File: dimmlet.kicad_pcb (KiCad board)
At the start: 2 copper layers, 204 x 20 mm, 23 parts, among them J1 Conn_01x02, J2 Conn_01x02, J3 CONN288_2-2308107-0_TEC, J4 Conn_01x06, J5 Conn_01x02, J6 Conn_01x02, J7 CONN288_2-2308107-0_TEC, U1 ‎TXS0102, U2 ‎MIC5365-2.5YC5-TR

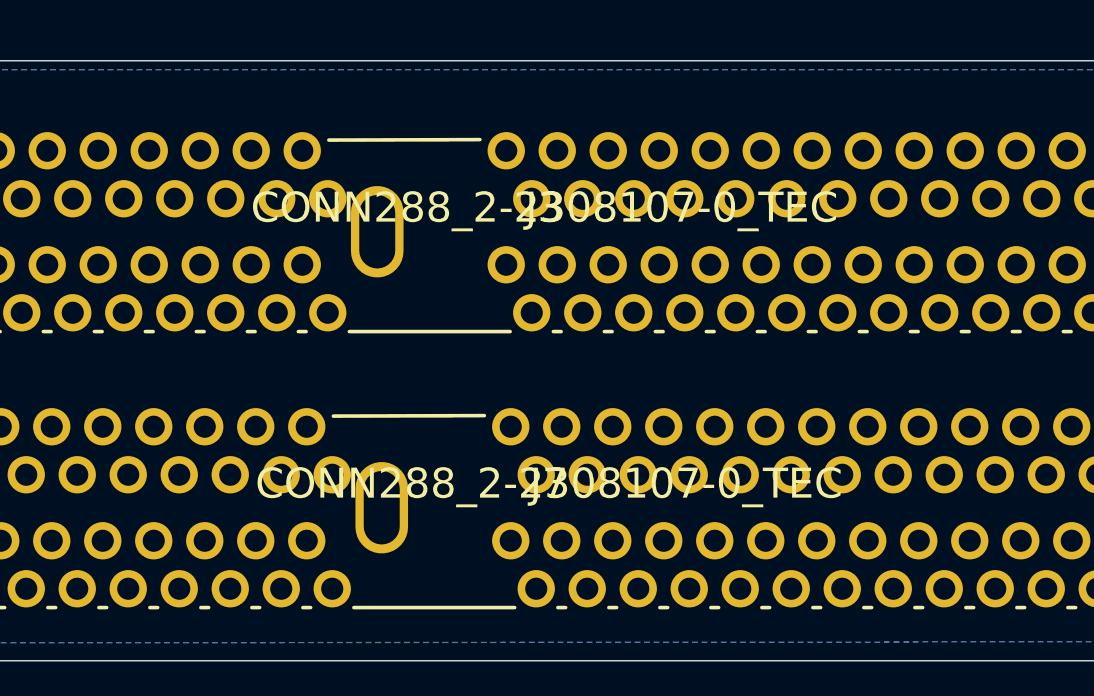
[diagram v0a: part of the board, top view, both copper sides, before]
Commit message: update
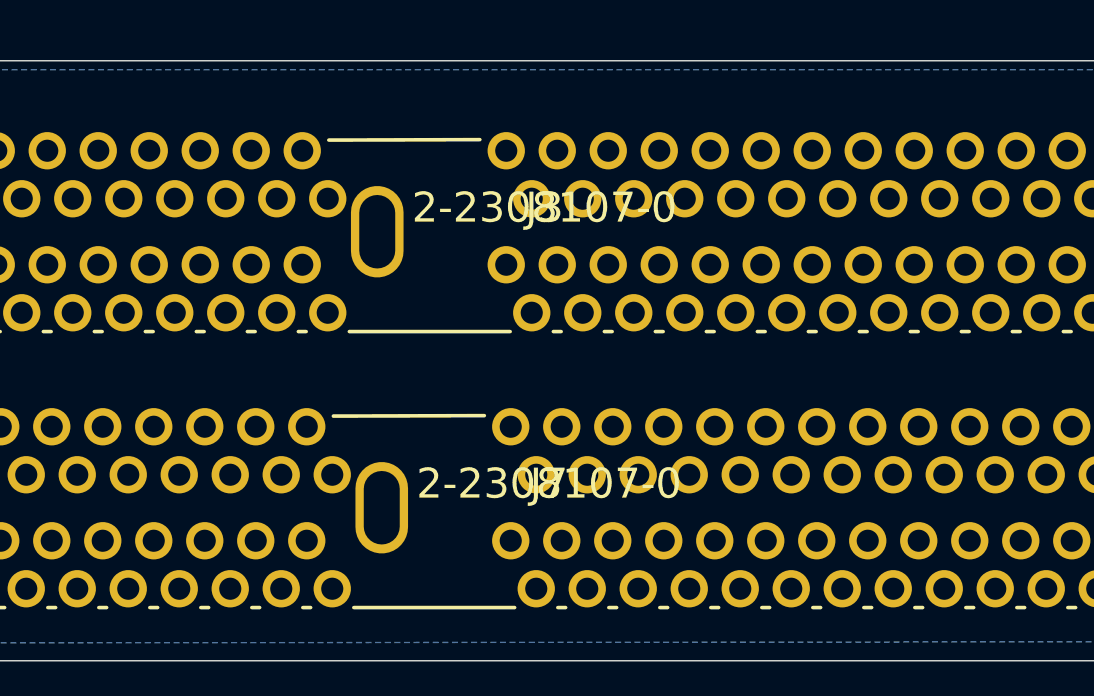
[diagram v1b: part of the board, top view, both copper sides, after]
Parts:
- J3, J7: value CONN288_2-2308107-0_TEC -> 2-2308107-0
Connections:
- J3 pad 1: Net-(J3-Pad1) -> unconnected-(J3-Pad1)
- J3 pad 10: Net-(J3-Pad10) -> unconnected-(J3-Pad10)
- J3 pad 100: Net-(J3-Pad100) -> unconnected-(J3-Pad100)
- J3 pad 102: Net-(J3-Pad102) -> unconnected-(J3-Pad102)
- J3 pad 104: Net-(J3-Pad104) -> unconnected-(J3-Pad104)
- J3 pad 106: Net-(J3-Pad106) -> unconnected-(J3-Pad106)
- J3 pad 108: Net-(J3-Pad108) -> unconnected-(J3-Pad108)
- J3 pad 110: Net-(J3-Pad110) -> unconnected-(J3-Pad110)
- J3 pad 111: Net-(J3-Pad111) -> unconnected-(J3-Pad111)
- J3 pad 113: Net-(J3-Pad113) -> unconnected-(J3-Pad113)
- J3 pad 115: Net-(J3-Pad115) -> unconnected-(J3-Pad115)
- J3 pad 117: Net-(J3-Pad117) -> unconnected-(J3-Pad117)
- J3 pad 119: Net-(J3-Pad119) -> unconnected-(J3-Pad119)
- J3 pad 12: Net-(J3-Pad12) -> unconnected-(J3-Pad12)
- J3 pad 121: Net-(J3-Pad121) -> unconnected-(J3-Pad121)
- J3 pad 122: Net-(J3-Pad122) -> unconnected-(J3-Pad122)
- J3 pad 124: Net-(J3-Pad124) -> unconnected-(J3-Pad124)
- J3 pad 126: Net-(J3-Pad126) -> unconnected-(J3-Pad126)
- J3 pad 128: Net-(J3-Pad128) -> unconnected-(J3-Pad128)
- J3 pad 130: Net-(J3-Pad130) -> unconnected-(J3-Pad130)
- J3 pad 132: Net-(J3-Pad132) -> unconnected-(J3-Pad132)
- J3 pad 133: Net-(J3-Pad133) -> unconnected-(J3-Pad133)
- J3 pad 135: Net-(J3-Pad135) -> unconnected-(J3-Pad135)
- J3 pad 137: Net-(J3-Pad137) -> unconnected-(J3-Pad137)
- J3 pad 14: Net-(J3-Pad14) -> unconnected-(J3-Pad14)
- J3 pad 142: Net-(J3-Pad142) -> unconnected-(J3-Pad142)
- J3 pad 143: Net-(J3-Pad143) -> unconnected-(J3-Pad143)
- J3 pad 144: Net-(J3-Pad144) -> unconnected-(J3-Pad144)
- J3 pad 145: Net-(J3-Pad145) -> unconnected-(J3-Pad145)
- J3 pad 146: Net-(J3-Pad146) -> unconnected-(J3-Pad146)
- J3 pad 148: Net-(J3-Pad148) -> unconnected-(J3-Pad148)
- J3 pad 150: Net-(J3-Pad150) -> unconnected-(J3-Pad150)
- J3 pad 152: Net-(J3-Pad152) -> unconnected-(J3-Pad152)
- J3 pad 153: Net-(J3-Pad153) -> unconnected-(J3-Pad153)
- J3 pad 155: Net-(J3-Pad155) -> unconnected-(J3-Pad155)
- J3 pad 157: Net-(J3-Pad157) -> unconnected-(J3-Pad157)
- J3 pad 159: Net-(J3-Pad159) -> unconnected-(J3-Pad159)
- J3 pad 16: Net-(J3-Pad16) -> unconnected-(J3-Pad16)
- J3 pad 161: Net-(J3-Pad161) -> unconnected-(J3-Pad161)
- J3 pad 163: Net-(J3-Pad163) -> unconnected-(J3-Pad163)
- J3 pad 164: Net-(J3-Pad164) -> unconnected-(J3-Pad164)
- J3 pad 166: Net-(J3-Pad166) -> unconnected-(J3-Pad166)
- J3 pad 168: Net-(J3-Pad168) -> unconnected-(J3-Pad168)
- J3 pad 170: Net-(J3-Pad170) -> unconnected-(J3-Pad170)
- J3 pad 172: Net-(J3-Pad172) -> unconnected-(J3-Pad172)
- J3 pad 174: Net-(J3-Pad174) -> unconnected-(J3-Pad174)
- J3 pad 175: Net-(J3-Pad175) -> unconnected-(J3-Pad175)
- J3 pad 177: Net-(J3-Pad177) -> unconnected-(J3-Pad177)
- J3 pad 179: Net-(J3-Pad179) -> unconnected-(J3-Pad179)
- J3 pad 18: Net-(J3-Pad18) -> unconnected-(J3-Pad18)
- J3 pad 181: Net-(J3-Pad181) -> unconnected-(J3-Pad181)
- J3 pad 183: Net-(J3-Pad183) -> unconnected-(J3-Pad183)
- J3 pad 185: Net-(J3-Pad185) -> unconnected-(J3-Pad185)
- J3 pad 186: Net-(J3-Pad186) -> unconnected-(J3-Pad186)
- J3 pad 188: Net-(J3-Pad188) -> unconnected-(J3-Pad188)
- J3 pad 19: Net-(J3-Pad19) -> unconnected-(J3-Pad19)
- J3 pad 190: Net-(J3-Pad190) -> unconnected-(J3-Pad190)
- J3 pad 192: Net-(J3-Pad192) -> unconnected-(J3-Pad192)
- J3 pad 194: Net-(J3-Pad194) -> unconnected-(J3-Pad194)
- J3 pad 196: Net-(J3-Pad196) -> unconnected-(J3-Pad196)
- J3 pad 197: Net-(J3-Pad197) -> unconnected-(J3-Pad197)
- J3 pad 199: Net-(J3-Pad199) -> unconnected-(J3-Pad199)
- J3 pad 201: Net-(J3-Pad201) -> unconnected-(J3-Pad201)
- J3 pad 203: Net-(J3-Pad203) -> unconnected-(J3-Pad203)
- J3 pad 204: Net-(J3-Pad204) -> unconnected-(J3-Pad204)
- J3 pad 205: Net-(J3-Pad205) -> unconnected-(J3-Pad205)
- J3 pad 206: Net-(J3-Pad206) -> unconnected-(J3-Pad206)
- J3 pad 207: Net-(J3-Pad207) -> unconnected-(J3-Pad207)
- J3 pad 208: Net-(J3-Pad208) -> unconnected-(J3-Pad208)
- J3 pad 209: Net-(J3-Pad209) -> unconnected-(J3-Pad209)
- J3 pad 21: Net-(J3-Pad21) -> unconnected-(J3-Pad21)
- J3 pad 210: Net-(J3-Pad210) -> unconnected-(J3-Pad210)
- J3 pad 211: Net-(J3-Pad211) -> unconnected-(J3-Pad211)
- J3 pad 212: Net-(J3-Pad212) -> unconnected-(J3-Pad212)
- J3 pad 213: Net-(J3-Pad213) -> unconnected-(J3-Pad213)
- J3 pad 214: Net-(J3-Pad214) -> unconnected-(J3-Pad214)
- J3 pad 215: Net-(J3-Pad215) -> unconnected-(J3-Pad215)
- J3 pad 216: Net-(J3-Pad216) -> unconnected-(J3-Pad216)
- J3 pad 217: Net-(J3-Pad217) -> unconnected-(J3-Pad217)
- J3 pad 218: Net-(J3-Pad218) -> unconnected-(J3-Pad218)
- J3 pad 219: Net-(J3-Pad219) -> unconnected-(J3-Pad219)
- J3 pad 220: Net-(J3-Pad220) -> unconnected-(J3-Pad220)
- J3 pad 221: Net-(J3-Pad221) -> unconnected-(J3-Pad221)
- J3 pad 222: Net-(J3-Pad222) -> unconnected-(J3-Pad222)
- J3 pad 223: Net-(J3-Pad223) -> unconnected-(J3-Pad223)
- J3 pad 224: Net-(J3-Pad224) -> unconnected-(J3-Pad224)
- J3 pad 225: Net-(J3-Pad225) -> unconnected-(J3-Pad225)
- J3 pad 226: Net-(J3-Pad226) -> unconnected-(J3-Pad226)
- J3 pad 227: Net-(J3-Pad227) -> unconnected-(J3-Pad227)
- J3 pad 228: Net-(J3-Pad228) -> unconnected-(J3-Pad228)
- J3 pad 229: Net-(J3-Pad229) -> unconnected-(J3-Pad229)
- J3 pad 23: Net-(J3-Pad23) -> unconnected-(J3-Pad23)
- J3 pad 230: Net-(J3-Pad230) -> unconnected-(J3-Pad230)
- J3 pad 231: Net-(J3-Pad231) -> unconnected-(J3-Pad231)
- J3 pad 232: Net-(J3-Pad232) -> unconnected-(J3-Pad232)
- J3 pad 233: Net-(J3-Pad233) -> unconnected-(J3-Pad233)
- J3 pad 234: Net-(J3-Pad234) -> unconnected-(J3-Pad234)
- J3 pad 235: Net-(J3-Pad235) -> unconnected-(J3-Pad235)
- J3 pad 236: Net-(J3-Pad236) -> unconnected-(J3-Pad236)
- J3 pad 237: Net-(J3-Pad237) -> unconnected-(J3-Pad237)
- J3 pad 238: Net-(J3-Pad238) -> unconnected-(J3-Pad238)
- J3 pad 240: Net-(J3-Pad240) -> unconnected-(J3-Pad240)
- J3 pad 242: Net-(J3-Pad242) -> unconnected-(J3-Pad242)
- J3 pad 244: Net-(J3-Pad244) -> unconnected-(J3-Pad244)
- J3 pad 245: Net-(J3-Pad245) -> unconnected-(J3-Pad245)
- J3 pad 247: Net-(J3-Pad247) -> unconnected-(J3-Pad247)
- J3 pad 249: Net-(J3-Pad249) -> unconnected-(J3-Pad249)
- J3 pad 25: Net-(J3-Pad25) -> unconnected-(J3-Pad25)
- J3 pad 251: Net-(J3-Pad251) -> unconnected-(J3-Pad251)
- J3 pad 253: Net-(J3-Pad253) -> unconnected-(J3-Pad253)
- J3 pad 255: Net-(J3-Pad255) -> unconnected-(J3-Pad255)
- J3 pad 256: Net-(J3-Pad256) -> unconnected-(J3-Pad256)
- J3 pad 258: Net-(J3-Pad258) -> unconnected-(J3-Pad258)
- J3 pad 260: Net-(J3-Pad260) -> unconnected-(J3-Pad260)
- J3 pad 262: Net-(J3-Pad262) -> unconnected-(J3-Pad262)
- J3 pad 264: Net-(J3-Pad264) -> unconnected-(J3-Pad264)
- J3 pad 266: Net-(J3-Pad266) -> unconnected-(J3-Pad266)
- J3 pad 267: Net-(J3-Pad267) -> unconnected-(J3-Pad267)
- J3 pad 269: Net-(J3-Pad269) -> unconnected-(J3-Pad269)
- J3 pad 27: Net-(J3-Pad27) -> unconnected-(J3-Pad27)
- J3 pad 271: Net-(J3-Pad271) -> unconnected-(J3-Pad271)
- J3 pad 273: Net-(J3-Pad273) -> unconnected-(J3-Pad273)
- J3 pad 275: Net-(J3-Pad275) -> unconnected-(J3-Pad275)
- J3 pad 277: Net-(J3-Pad277) -> unconnected-(J3-Pad277)
- J3 pad 278: Net-(J3-Pad278) -> unconnected-(J3-Pad278)
- J3 pad 280: Net-(J3-Pad280) -> unconnected-(J3-Pad280)
- J3 pad 282: Net-(J3-Pad282) -> unconnected-(J3-Pad282)
- J3 pad 286: Net-(J3-Pad286) -> unconnected-(J3-Pad286)
- J3 pad 287: Net-(J3-Pad287) -> unconnected-(J3-Pad287)
- J3 pad 288: Net-(J3-Pad288) -> unconnected-(J3-Pad288)
- J3 pad 29: Net-(J3-Pad29) -> unconnected-(J3-Pad29)
- J3 pad 3: Net-(J3-Pad3) -> unconnected-(J3-Pad3)
- J3 pad 30: Net-(J3-Pad30) -> unconnected-(J3-Pad30)
- J3 pad 32: Net-(J3-Pad32) -> unconnected-(J3-Pad32)
- J3 pad 34: Net-(J3-Pad34) -> unconnected-(J3-Pad34)
- J3 pad 36: Net-(J3-Pad36) -> unconnected-(J3-Pad36)
- J3 pad 38: Net-(J3-Pad38) -> unconnected-(J3-Pad38)
- J3 pad 40: Net-(J3-Pad40) -> unconnected-(J3-Pad40)
- J3 pad 41: Net-(J3-Pad41) -> unconnected-(J3-Pad41)
- J3 pad 43: Net-(J3-Pad43) -> unconnected-(J3-Pad43)
- J3 pad 45: Net-(J3-Pad45) -> unconnected-(J3-Pad45)
- J3 pad 47: Net-(J3-Pad47) -> unconnected-(J3-Pad47)
- J3 pad 49: Net-(J3-Pad49) -> unconnected-(J3-Pad49)
- J3 pad 5: Net-(J3-Pad5) -> unconnected-(J3-Pad5)
- J3 pad 51: Net-(J3-Pad51) -> unconnected-(J3-Pad51)
- J3 pad 52: Net-(J3-Pad52) -> unconnected-(J3-Pad52)
- J3 pad 54: Net-(J3-Pad54) -> unconnected-(J3-Pad54)
- J3 pad 56: Net-(J3-Pad56) -> unconnected-(J3-Pad56)
- J3 pad 58: Net-(J3-Pad58) -> unconnected-(J3-Pad58)
- J3 pad 59: Net-(J3-Pad59) -> unconnected-(J3-Pad59)
- J3 pad 60: Net-(J3-Pad60) -> unconnected-(J3-Pad60)
- J3 pad 61: Net-(J3-Pad61) -> unconnected-(J3-Pad61)
- J3 pad 62: Net-(J3-Pad62) -> unconnected-(J3-Pad62)
- J3 pad 63: Net-(J3-Pad63) -> unconnected-(J3-Pad63)
- J3 pad 64: Net-(J3-Pad64) -> unconnected-(J3-Pad64)
- J3 pad 65: Net-(J3-Pad65) -> unconnected-(J3-Pad65)
- J3 pad 66: Net-(J3-Pad66) -> unconnected-(J3-Pad66)
- J3 pad 67: Net-(J3-Pad67) -> unconnected-(J3-Pad67)
- J3 pad 68: Net-(J3-Pad68) -> unconnected-(J3-Pad68)
- J3 pad 69: Net-(J3-Pad69) -> unconnected-(J3-Pad69)
- J3 pad 7: Net-(J3-Pad7) -> unconnected-(J3-Pad7)
- J3 pad 70: Net-(J3-Pad70) -> unconnected-(J3-Pad70)
- J3 pad 71: Net-(J3-Pad71) -> unconnected-(J3-Pad71)
- J3 pad 72: Net-(J3-Pad72) -> unconnected-(J3-Pad72)
- J3 pad 73: Net-(J3-Pad73) -> unconnected-(J3-Pad73)
- J3 pad 74: Net-(J3-Pad74) -> unconnected-(J3-Pad74)
- J3 pad 75: Net-(J3-Pad75) -> unconnected-(J3-Pad75)
- J3 pad 76: Net-(J3-Pad76) -> unconnected-(J3-Pad76)
- J3 pad 77: Net-(J3-Pad77) -> unconnected-(J3-Pad77)
- J3 pad 78: Net-(J3-Pad78) -> unconnected-(J3-Pad78)
- J3 pad 79: Net-(J3-Pad79) -> unconnected-(J3-Pad79)
- J3 pad 8: Net-(J3-Pad8) -> unconnected-(J3-Pad8)
- J3 pad 80: Net-(J3-Pad80) -> unconnected-(J3-Pad80)
- J3 pad 81: Net-(J3-Pad81) -> unconnected-(J3-Pad81)
- J3 pad 82: Net-(J3-Pad82) -> unconnected-(J3-Pad82)
- J3 pad 83: Net-(J3-Pad83) -> unconnected-(J3-Pad83)
- J3 pad 84: Net-(J3-Pad84) -> unconnected-(J3-Pad84)
- J3 pad 85: Net-(J3-Pad85) -> unconnected-(J3-Pad85)
- J3 pad 86: Net-(J3-Pad86) -> unconnected-(J3-Pad86)
- J3 pad 87: Net-(J3-Pad87) -> unconnected-(J3-Pad87)
- J3 pad 88: Net-(J3-Pad88) -> unconnected-(J3-Pad88)
- J3 pad 89: Net-(J3-Pad89) -> unconnected-(J3-Pad89)
- J3 pad 90: Net-(J3-Pad90) -> unconnected-(J3-Pad90)
- J3 pad 91: Net-(J3-Pad91) -> unconnected-(J3-Pad91)
- J3 pad 92: Net-(J3-Pad92) -> unconnected-(J3-Pad92)
- J3 pad 93: Net-(J3-Pad93) -> unconnected-(J3-Pad93)
- J3 pad 95: Net-(J3-Pad95) -> unconnected-(J3-Pad95)
- J3 pad 97: Net-(J3-Pad97) -> unconnected-(J3-Pad97)
- J3 pad 99: Net-(J3-Pad99) -> unconnected-(J3-Pad99)
- J4 pad 1: Net-(J4-Pad1) -> unconnected-(J4-Pin_1-Pad1)
- J4 pad 2: Net-(J4-Pad2) -> unconnected-(J4-Pin_2-Pad2)
- J7 pad 1: Net-(J7-Pad1) -> unconnected-(J7-Pad1)
- J7 pad 10: Net-(J7-Pad10) -> unconnected-(J7-Pad10)
- J7 pad 100: Net-(J7-Pad100) -> unconnected-(J7-Pad100)
- J7 pad 102: Net-(J7-Pad102) -> unconnected-(J7-Pad102)
- J7 pad 104: Net-(J7-Pad104) -> unconnected-(J7-Pad104)
- J7 pad 106: Net-(J7-Pad106) -> unconnected-(J7-Pad106)
- J7 pad 108: Net-(J7-Pad108) -> unconnected-(J7-Pad108)
- J7 pad 110: Net-(J7-Pad110) -> unconnected-(J7-Pad110)
- J7 pad 111: Net-(J7-Pad111) -> unconnected-(J7-Pad111)
- J7 pad 113: Net-(J7-Pad113) -> unconnected-(J7-Pad113)
- J7 pad 115: Net-(J7-Pad115) -> unconnected-(J7-Pad115)
- J7 pad 117: Net-(J7-Pad117) -> unconnected-(J7-Pad117)
- J7 pad 119: Net-(J7-Pad119) -> unconnected-(J7-Pad119)
- J7 pad 12: Net-(J7-Pad12) -> unconnected-(J7-Pad12)
- J7 pad 121: Net-(J7-Pad121) -> unconnected-(J7-Pad121)
- J7 pad 122: Net-(J7-Pad122) -> unconnected-(J7-Pad122)
- J7 pad 124: Net-(J7-Pad124) -> unconnected-(J7-Pad124)
- J7 pad 126: Net-(J7-Pad126) -> unconnected-(J7-Pad126)
- J7 pad 128: Net-(J7-Pad128) -> unconnected-(J7-Pad128)
- J7 pad 130: Net-(J7-Pad130) -> unconnected-(J7-Pad130)
- J7 pad 132: Net-(J7-Pad132) -> unconnected-(J7-Pad132)
- J7 pad 133: Net-(J7-Pad133) -> unconnected-(J7-Pad133)
- J7 pad 135: Net-(J7-Pad135) -> unconnected-(J7-Pad135)
- J7 pad 137: Net-(J7-Pad137) -> unconnected-(J7-Pad137)
- J7 pad 14: Net-(J7-Pad14) -> unconnected-(J7-Pad14)
- J7 pad 142: Net-(J7-Pad142) -> unconnected-(J7-Pad142)
- J7 pad 143: Net-(J7-Pad143) -> unconnected-(J7-Pad143)
- J7 pad 144: Net-(J7-Pad144) -> unconnected-(J7-Pad144)
- J7 pad 145: Net-(J7-Pad145) -> unconnected-(J7-Pad145)
- J7 pad 146: Net-(J7-Pad146) -> unconnected-(J7-Pad146)
- J7 pad 148: Net-(J7-Pad148) -> unconnected-(J7-Pad148)
- J7 pad 150: Net-(J7-Pad150) -> unconnected-(J7-Pad150)
- J7 pad 152: Net-(J7-Pad152) -> unconnected-(J7-Pad152)
- J7 pad 153: Net-(J7-Pad153) -> unconnected-(J7-Pad153)
- J7 pad 155: Net-(J7-Pad155) -> unconnected-(J7-Pad155)
- J7 pad 157: Net-(J7-Pad157) -> unconnected-(J7-Pad157)
- J7 pad 159: Net-(J7-Pad159) -> unconnected-(J7-Pad159)
- J7 pad 16: Net-(J7-Pad16) -> unconnected-(J7-Pad16)
- J7 pad 161: Net-(J7-Pad161) -> unconnected-(J7-Pad161)
- J7 pad 163: Net-(J7-Pad163) -> unconnected-(J7-Pad163)
- J7 pad 164: Net-(J7-Pad164) -> unconnected-(J7-Pad164)
- J7 pad 166: Net-(J7-Pad166) -> unconnected-(J7-Pad166)
- J7 pad 168: Net-(J7-Pad168) -> unconnected-(J7-Pad168)
- J7 pad 170: Net-(J7-Pad170) -> unconnected-(J7-Pad170)
- J7 pad 172: Net-(J7-Pad172) -> unconnected-(J7-Pad172)
- J7 pad 174: Net-(J7-Pad174) -> unconnected-(J7-Pad174)
- J7 pad 175: Net-(J7-Pad175) -> unconnected-(J7-Pad175)
- J7 pad 177: Net-(J7-Pad177) -> unconnected-(J7-Pad177)
- J7 pad 179: Net-(J7-Pad179) -> unconnected-(J7-Pad179)
- J7 pad 18: Net-(J7-Pad18) -> unconnected-(J7-Pad18)
- J7 pad 181: Net-(J7-Pad181) -> unconnected-(J7-Pad181)
- J7 pad 183: Net-(J7-Pad183) -> unconnected-(J7-Pad183)
- J7 pad 185: Net-(J7-Pad185) -> unconnected-(J7-Pad185)
- J7 pad 186: Net-(J7-Pad186) -> unconnected-(J7-Pad186)
- J7 pad 188: Net-(J7-Pad188) -> unconnected-(J7-Pad188)
- J7 pad 19: Net-(J7-Pad19) -> unconnected-(J7-Pad19)
- J7 pad 190: Net-(J7-Pad190) -> unconnected-(J7-Pad190)
- J7 pad 192: Net-(J7-Pad192) -> unconnected-(J7-Pad192)
- J7 pad 194: Net-(J7-Pad194) -> unconnected-(J7-Pad194)
- J7 pad 196: Net-(J7-Pad196) -> unconnected-(J7-Pad196)
- J7 pad 197: Net-(J7-Pad197) -> unconnected-(J7-Pad197)
- J7 pad 199: Net-(J7-Pad199) -> unconnected-(J7-Pad199)
- J7 pad 201: Net-(J7-Pad201) -> unconnected-(J7-Pad201)
- J7 pad 203: Net-(J7-Pad203) -> unconnected-(J7-Pad203)
- J7 pad 204: Net-(J7-Pad204) -> unconnected-(J7-Pad204)
- J7 pad 205: Net-(J7-Pad205) -> unconnected-(J7-Pad205)
- J7 pad 206: Net-(J7-Pad206) -> unconnected-(J7-Pad206)
- J7 pad 207: Net-(J7-Pad207) -> unconnected-(J7-Pad207)
- J7 pad 208: Net-(J7-Pad208) -> unconnected-(J7-Pad208)
- J7 pad 209: Net-(J7-Pad209) -> unconnected-(J7-Pad209)
- J7 pad 21: Net-(J7-Pad21) -> unconnected-(J7-Pad21)
- J7 pad 210: Net-(J7-Pad210) -> unconnected-(J7-Pad210)
- J7 pad 211: Net-(J7-Pad211) -> unconnected-(J7-Pad211)
- J7 pad 212: Net-(J7-Pad212) -> unconnected-(J7-Pad212)
- J7 pad 213: Net-(J7-Pad213) -> unconnected-(J7-Pad213)
- J7 pad 214: Net-(J7-Pad214) -> unconnected-(J7-Pad214)
- J7 pad 215: Net-(J7-Pad215) -> unconnected-(J7-Pad215)
- J7 pad 216: Net-(J7-Pad216) -> unconnected-(J7-Pad216)
- J7 pad 217: Net-(J7-Pad217) -> unconnected-(J7-Pad217)
- J7 pad 218: Net-(J7-Pad218) -> unconnected-(J7-Pad218)
- J7 pad 219: Net-(J7-Pad219) -> unconnected-(J7-Pad219)
- J7 pad 220: Net-(J7-Pad220) -> unconnected-(J7-Pad220)
- J7 pad 221: Net-(J7-Pad221) -> unconnected-(J7-Pad221)
- J7 pad 222: Net-(J7-Pad222) -> unconnected-(J7-Pad222)
- J7 pad 223: Net-(J7-Pad223) -> unconnected-(J7-Pad223)
- J7 pad 224: Net-(J7-Pad224) -> unconnected-(J7-Pad224)
- J7 pad 225: Net-(J7-Pad225) -> unconnected-(J7-Pad225)
- J7 pad 226: Net-(J7-Pad226) -> unconnected-(J7-Pad226)
- J7 pad 227: Net-(J7-Pad227) -> unconnected-(J7-Pad227)
- J7 pad 228: Net-(J7-Pad228) -> unconnected-(J7-Pad228)
- J7 pad 229: Net-(J7-Pad229) -> unconnected-(J7-Pad229)
- J7 pad 23: Net-(J7-Pad23) -> unconnected-(J7-Pad23)
- J7 pad 230: Net-(J7-Pad230) -> unconnected-(J7-Pad230)
- J7 pad 231: Net-(J7-Pad231) -> unconnected-(J7-Pad231)
- J7 pad 232: Net-(J7-Pad232) -> unconnected-(J7-Pad232)
- J7 pad 233: Net-(J7-Pad233) -> unconnected-(J7-Pad233)
- J7 pad 234: Net-(J7-Pad234) -> unconnected-(J7-Pad234)
- J7 pad 235: Net-(J7-Pad235) -> unconnected-(J7-Pad235)
- J7 pad 236: Net-(J7-Pad236) -> unconnected-(J7-Pad236)
- J7 pad 237: Net-(J7-Pad237) -> unconnected-(J7-Pad237)
- J7 pad 238: Net-(J7-Pad238) -> unconnected-(J7-Pad238)
- J7 pad 240: Net-(J7-Pad240) -> unconnected-(J7-Pad240)
- J7 pad 242: Net-(J7-Pad242) -> unconnected-(J7-Pad242)
- J7 pad 244: Net-(J7-Pad244) -> unconnected-(J7-Pad244)
- J7 pad 245: Net-(J7-Pad245) -> unconnected-(J7-Pad245)
- J7 pad 247: Net-(J7-Pad247) -> unconnected-(J7-Pad247)
- J7 pad 249: Net-(J7-Pad249) -> unconnected-(J7-Pad249)
- J7 pad 25: Net-(J7-Pad25) -> unconnected-(J7-Pad25)
- J7 pad 251: Net-(J7-Pad251) -> unconnected-(J7-Pad251)
- J7 pad 253: Net-(J7-Pad253) -> unconnected-(J7-Pad253)
- J7 pad 255: Net-(J7-Pad255) -> unconnected-(J7-Pad255)
- J7 pad 256: Net-(J7-Pad256) -> unconnected-(J7-Pad256)
- J7 pad 258: Net-(J7-Pad258) -> unconnected-(J7-Pad258)
- J7 pad 260: Net-(J7-Pad260) -> unconnected-(J7-Pad260)
- J7 pad 262: Net-(J7-Pad262) -> unconnected-(J7-Pad262)
- J7 pad 264: Net-(J7-Pad264) -> unconnected-(J7-Pad264)
- J7 pad 266: Net-(J7-Pad266) -> unconnected-(J7-Pad266)
- J7 pad 267: Net-(J7-Pad267) -> unconnected-(J7-Pad267)
- J7 pad 269: Net-(J7-Pad269) -> unconnected-(J7-Pad269)
- J7 pad 27: Net-(J7-Pad27) -> unconnected-(J7-Pad27)
- J7 pad 271: Net-(J7-Pad271) -> unconnected-(J7-Pad271)
- J7 pad 273: Net-(J7-Pad273) -> unconnected-(J7-Pad273)
- J7 pad 275: Net-(J7-Pad275) -> unconnected-(J7-Pad275)
- J7 pad 277: Net-(J7-Pad277) -> unconnected-(J7-Pad277)
- J7 pad 278: Net-(J7-Pad278) -> unconnected-(J7-Pad278)
- J7 pad 280: Net-(J7-Pad280) -> unconnected-(J7-Pad280)
- J7 pad 282: Net-(J7-Pad282) -> unconnected-(J7-Pad282)
- J7 pad 286: Net-(J7-Pad286) -> unconnected-(J7-Pad286)
- J7 pad 287: Net-(J7-Pad287) -> unconnected-(J7-Pad287)
- J7 pad 288: Net-(J7-Pad288) -> unconnected-(J7-Pad288)
- J7 pad 29: Net-(J7-Pad29) -> unconnected-(J7-Pad29)
- J7 pad 3: Net-(J7-Pad3) -> unconnected-(J7-Pad3)
- J7 pad 30: Net-(J7-Pad30) -> unconnected-(J7-Pad30)
- J7 pad 32: Net-(J7-Pad32) -> unconnected-(J7-Pad32)
- J7 pad 34: Net-(J7-Pad34) -> unconnected-(J7-Pad34)
- J7 pad 36: Net-(J7-Pad36) -> unconnected-(J7-Pad36)
- J7 pad 38: Net-(J7-Pad38) -> unconnected-(J7-Pad38)
- J7 pad 40: Net-(J7-Pad40) -> unconnected-(J7-Pad40)
- J7 pad 41: Net-(J7-Pad41) -> unconnected-(J7-Pad41)
- J7 pad 43: Net-(J7-Pad43) -> unconnected-(J7-Pad43)
- J7 pad 45: Net-(J7-Pad45) -> unconnected-(J7-Pad45)
- J7 pad 47: Net-(J7-Pad47) -> unconnected-(J7-Pad47)
- J7 pad 49: Net-(J7-Pad49) -> unconnected-(J7-Pad49)
- J7 pad 5: Net-(J7-Pad5) -> unconnected-(J7-Pad5)
- J7 pad 51: Net-(J7-Pad51) -> unconnected-(J7-Pad51)
- J7 pad 52: Net-(J7-Pad52) -> unconnected-(J7-Pad52)
- J7 pad 54: Net-(J7-Pad54) -> unconnected-(J7-Pad54)
- J7 pad 56: Net-(J7-Pad56) -> unconnected-(J7-Pad56)
- J7 pad 58: Net-(J7-Pad58) -> unconnected-(J7-Pad58)
- J7 pad 59: Net-(J7-Pad59) -> unconnected-(J7-Pad59)
- J7 pad 60: Net-(J7-Pad60) -> unconnected-(J7-Pad60)
- J7 pad 61: Net-(J7-Pad61) -> unconnected-(J7-Pad61)
- J7 pad 62: Net-(J7-Pad62) -> unconnected-(J7-Pad62)
- J7 pad 63: Net-(J7-Pad63) -> unconnected-(J7-Pad63)
- J7 pad 64: Net-(J7-Pad64) -> unconnected-(J7-Pad64)
- J7 pad 65: Net-(J7-Pad65) -> unconnected-(J7-Pad65)
- J7 pad 66: Net-(J7-Pad66) -> unconnected-(J7-Pad66)
- J7 pad 67: Net-(J7-Pad67) -> unconnected-(J7-Pad67)
- J7 pad 68: Net-(J7-Pad68) -> unconnected-(J7-Pad68)
- J7 pad 69: Net-(J7-Pad69) -> unconnected-(J7-Pad69)
- J7 pad 7: Net-(J7-Pad7) -> unconnected-(J7-Pad7)
- J7 pad 70: Net-(J7-Pad70) -> unconnected-(J7-Pad70)
- J7 pad 71: Net-(J7-Pad71) -> unconnected-(J7-Pad71)
- J7 pad 72: Net-(J7-Pad72) -> unconnected-(J7-Pad72)
- J7 pad 73: Net-(J7-Pad73) -> unconnected-(J7-Pad73)
- J7 pad 74: Net-(J7-Pad74) -> unconnected-(J7-Pad74)
- J7 pad 75: Net-(J7-Pad75) -> unconnected-(J7-Pad75)
- J7 pad 76: Net-(J7-Pad76) -> unconnected-(J7-Pad76)
- J7 pad 77: Net-(J7-Pad77) -> unconnected-(J7-Pad77)
- J7 pad 78: Net-(J7-Pad78) -> unconnected-(J7-Pad78)
- J7 pad 79: Net-(J7-Pad79) -> unconnected-(J7-Pad79)
- J7 pad 8: Net-(J7-Pad8) -> unconnected-(J7-Pad8)
- J7 pad 80: Net-(J7-Pad80) -> unconnected-(J7-Pad80)
- J7 pad 81: Net-(J7-Pad81) -> unconnected-(J7-Pad81)
- J7 pad 82: Net-(J7-Pad82) -> unconnected-(J7-Pad82)
- J7 pad 83: Net-(J7-Pad83) -> unconnected-(J7-Pad83)
- J7 pad 84: Net-(J7-Pad84) -> unconnected-(J7-Pad84)
- J7 pad 85: Net-(J7-Pad85) -> unconnected-(J7-Pad85)
- J7 pad 86: Net-(J7-Pad86) -> unconnected-(J7-Pad86)
- J7 pad 87: Net-(J7-Pad87) -> unconnected-(J7-Pad87)
- J7 pad 88: Net-(J7-Pad88) -> unconnected-(J7-Pad88)
- J7 pad 89: Net-(J7-Pad89) -> unconnected-(J7-Pad89)
- J7 pad 90: Net-(J7-Pad90) -> unconnected-(J7-Pad90)
- J7 pad 91: Net-(J7-Pad91) -> unconnected-(J7-Pad91)
- J7 pad 92: Net-(J7-Pad92) -> unconnected-(J7-Pad92)
- J7 pad 93: Net-(J7-Pad93) -> unconnected-(J7-Pad93)
- J7 pad 95: Net-(J7-Pad95) -> unconnected-(J7-Pad95)
- J7 pad 97: Net-(J7-Pad97) -> unconnected-(J7-Pad97)
- J7 pad 99: Net-(J7-Pad99) -> unconnected-(J7-Pad99)
- U2 pad 4: Net-(U2-Pad4) -> unconnected-(U2-NC-Pad4)
